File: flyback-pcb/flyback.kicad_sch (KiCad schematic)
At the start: 10 parts, among them U1 CAP200DG, U2 CAP200DG

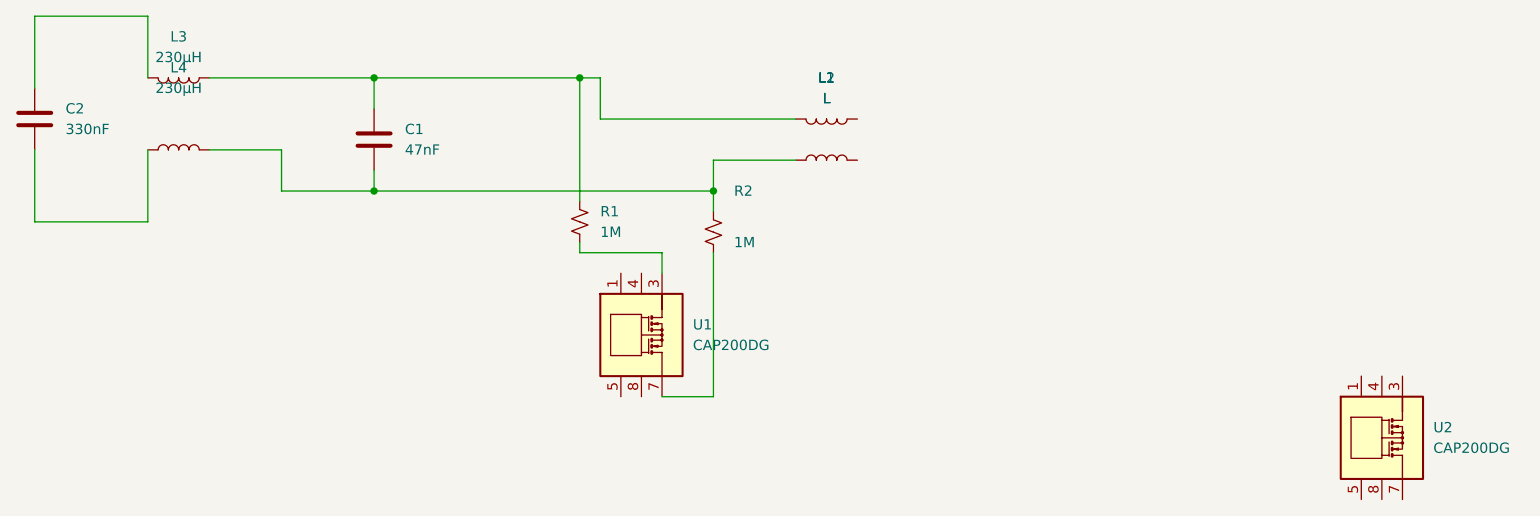
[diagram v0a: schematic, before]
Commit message: day2part2
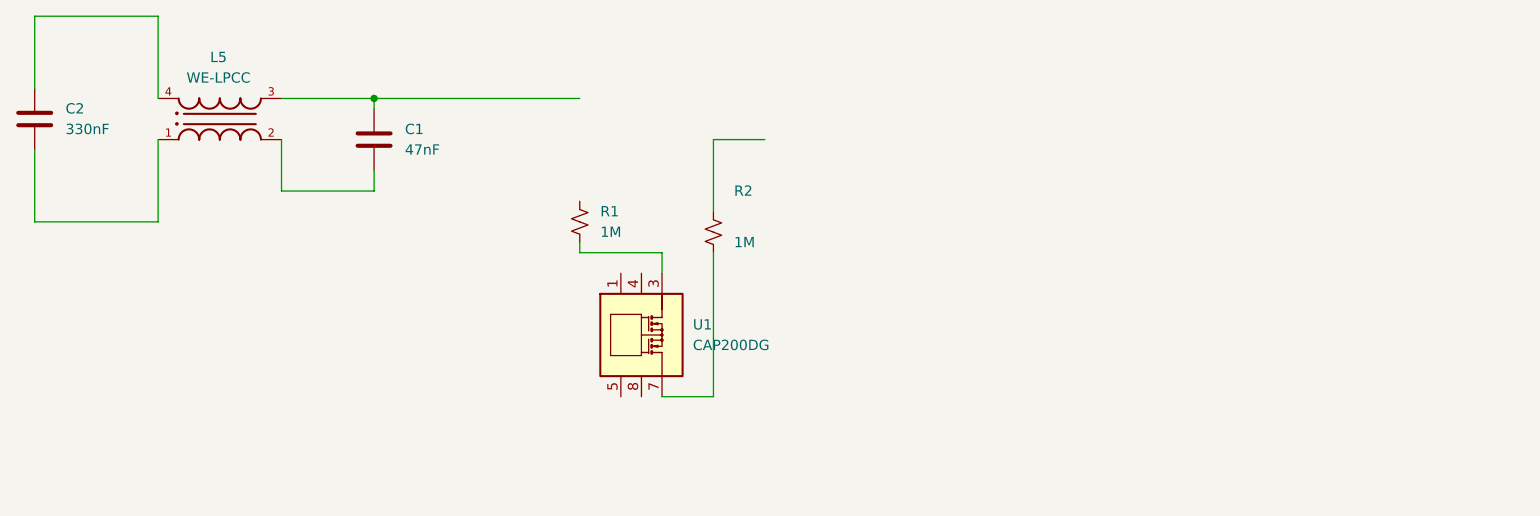
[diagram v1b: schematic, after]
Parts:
- removed L1, L2: L, symbol Device:L
- removed L3, L4: 230µH, symbol Device:L
- removed U2: CAP200DG, Package_SO:SOIC-8_3.9x4.9mm_P1.27mm, symbol Power_Management:CAP200DG
- added L5: WE-LPCC, WE-LPCC:WE-LPCC_7448680140, symbol WE-LPCC:WE-LPCC
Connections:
- net at R2.1: no longer C1.2
- net at C1.1: now also L5.3; no longer R1.1
- net at C2.1: now also L5.4
- net at C2.2: now also L5.1
- new net: C1.2, L5.2
